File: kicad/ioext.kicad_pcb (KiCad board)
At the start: 2 copper layers, 46 parts, among them P1 CONN_01X04, P2 CONN_02X08, P3 CONN_01X10, Q1 IRLZ44N, Q2 IRLZ44N, Q3 IRLZ44N, Q4 IRLZ44N, Q5 IRLZ44N, Q6 IRLZ44N, Q7 IRLZ44N, Q8 IRLZ44N, U1 PCF8574A, U2 PC817, U3 PC817, U4 PC817, U5 PC817, U6 PC817, U7 PC817, U8 PC817, U9 PC817

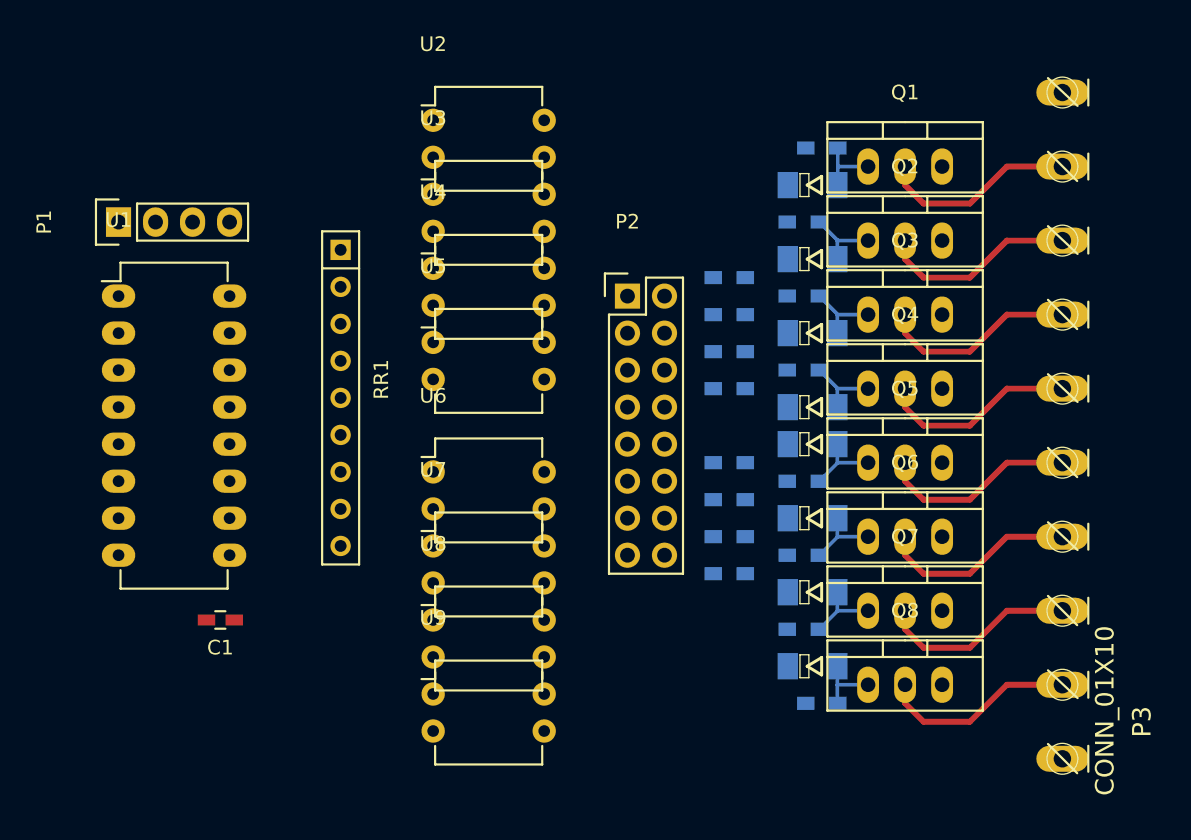
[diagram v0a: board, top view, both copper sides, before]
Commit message: kicad-ioext: wiring
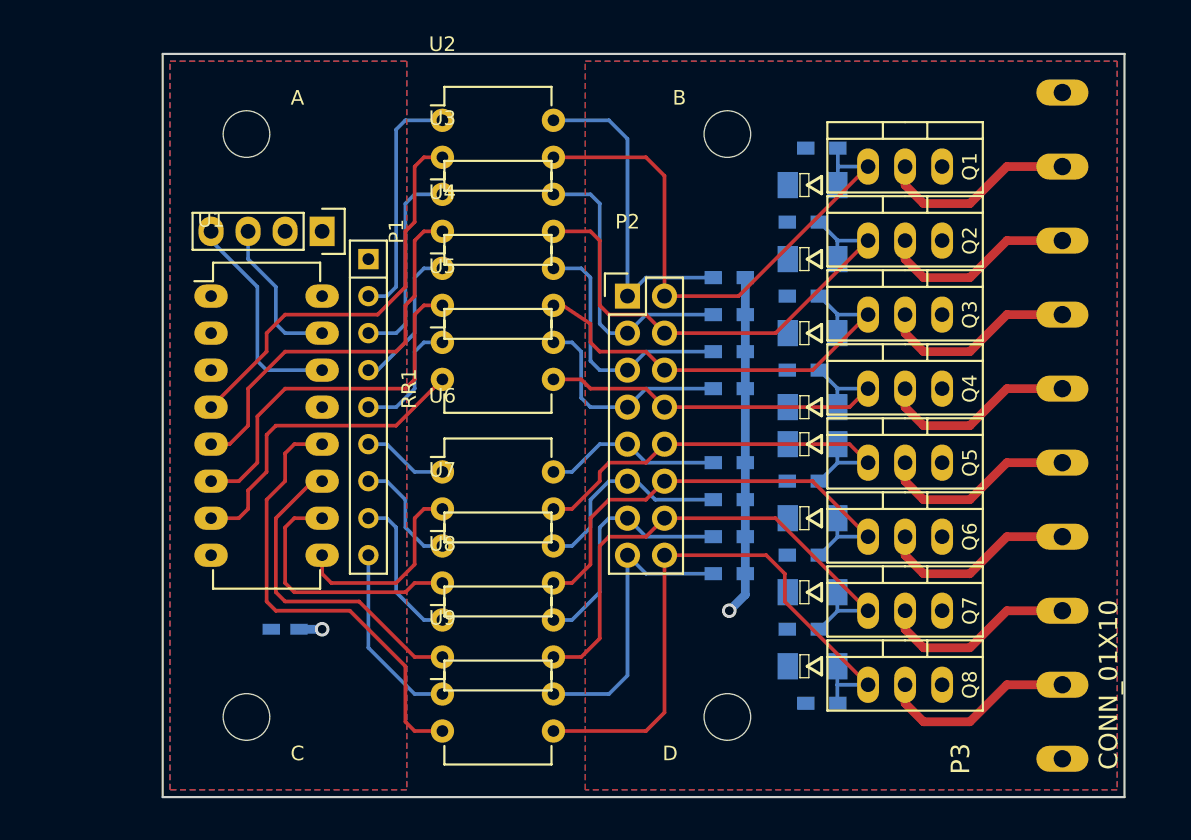
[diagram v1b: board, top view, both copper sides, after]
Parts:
- added A: MountingHole_3.2mm_M3, Mounting_Holes:MountingHole_3.2mm_M3, F.Cu at (213.2, 91.8)
- added B: MountingHole_3.2mm_M3, Mounting_Holes:MountingHole_3.2mm_M3, F.Cu at (246.2, 91.8)
- added C: MountingHole_3.2mm_M3, Mounting_Holes:MountingHole_3.2mm_M3, F.Cu at (213.2, 131.8)
- added D: MountingHole_3.2mm_M3, Mounting_Holes:MountingHole_3.2mm_M3, F.Cu at (246.2, 131.8)
- C1: moved to B.Cu
- moved P1 14.0 mm to (218.4, 98.4), turned to 270 degrees
- moved U1 6.35 mm to (210.8, 102.9)
- moved C1 4.49 mm to (215.9, 125.7)
- moved RR1 2.01 mm to (221.6, 110.5)
- moved U2 0.63 mm to (226.7, 90.8)
- moved U3 0.63 mm to (226.7, 95.9)
- moved U4 0.63 mm to (226.7, 101.0)
- moved U5 0.63 mm to (226.7, 106.0)
- moved U6 0.63 mm to (226.7, 114.9)
- moved U7 0.63 mm to (226.7, 120.0)
- moved U8 0.63 mm to (226.7, 125.1)
- moved U9 0.63 mm to (226.7, 130.2)
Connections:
- D6 pad 2: Net-(D6-Pad2) -> GNDA
- Q6 pad 3: GNDA -> Net-(Q6-Pad3)
- R14 pad 2: Net-(R14-Pad2) -> GNDA
- U1 pad 14: Net-(P1-Pad3) -> Net-(P1-Pad4)
- U1 pad 15: Net-(P1-Pad4) -> Net-(P1-Pad3)
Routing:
- net Net-(D8-Pad1): track 4.67 -> 42.4 mm
- net Net-(D1-Pad1): track 4.63 -> 38.7 mm
- net Net-(D7-Pad1): track 5.18 -> 37.1 mm
- net Net-(U1-Pad12): track 0.00 -> 31.5 mm
- net Net-(D2-Pad1): track 5.16 -> 34.9 mm
- net Net-(U1-Pad4): track 0.00 -> 28.2 mm
- net Net-(D6-Pad1): track 5.18 -> 33.1 mm
- net Net-(U1-Pad5): track 0.00 -> 27.1 mm
- net Net-(D3-Pad1): track 5.16 -> 30.8 mm
- net Net-(U1-Pad6): track 0.00 -> 25.3 mm
- net Net-(D5-Pad1): track 5.18 -> 29.5 mm
- net +12V: track 0.00 -> 23.3 mm, vias 0 -> 1
- net Net-(D4-Pad1): track 5.16 -> 28.1 mm
- net Net-(P2-Pad1): track 0.00 -> 22.8 mm
- net Net-(U1-Pad11): track 0.00 -> 22.6 mm
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- added copper zone on F.Cu, net +12V
- added copper zone on F.Cu, net +5V
- added copper zone on B.Cu, net GND
- added copper zone on B.Cu, net GNDA
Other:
- board outline added: 66 x 51 mm
- net class Default: trace_width 0.25 -> 0.254
- net class Power: trace_width 0.4 -> 0.6
